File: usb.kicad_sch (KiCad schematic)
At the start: 4 parts, among them J8 MC-121-L124, U6 USBLC6-2SC6

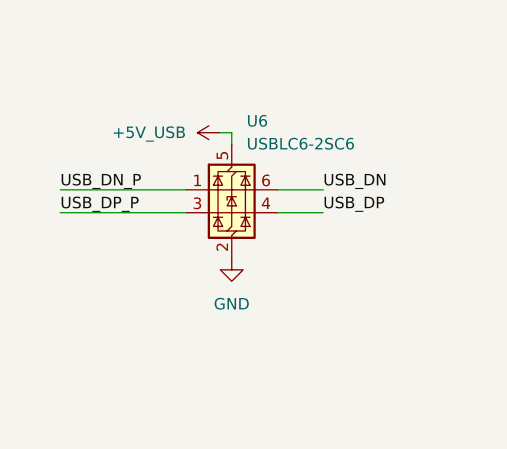
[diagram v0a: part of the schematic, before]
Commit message: Fix global nets
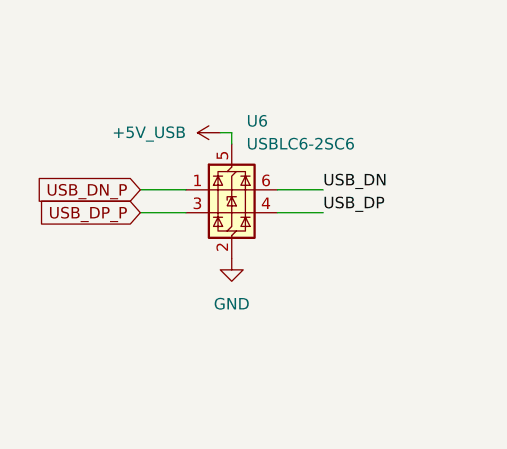
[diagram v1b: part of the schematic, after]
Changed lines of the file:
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@@
 	(wire
 		(pts
-			(xy 63.5 55.88) (xy 77.47 55.88)
+			(xy 72.39 53.34) (xy 77.47 53.34)
 		)
 		(stroke
@@
 		(pts
 			(xy 160.02 52.07) (xy 170.18 52.07)
+		)
+		(stroke
+			(width 0)
+			(type default)
+		)
+	)
+	(wire
+		(pts
+			(xy 72.39 55.88) (xy 77.47 55.88)
 		)
 		(stroke
@@
 	(wire
 		(pts
-			(xy 63.5 53.34) (xy 77.47 53.34)
-		)
-		(stroke
-			(width 0)
-			(type default)
-		)
-	)
-	(wire
-		(pts
 			(xy 168.91 69.85) (xy 168.91 67.31)
 		)
@@
 	(label "USB_DP"
 		(at 160.02 46.99 0)
-		(effects
-			(font
-				(size 1.27 1.27)
-			)
-			(justify left bottom)
-		)
-	)
-	(label "USB_DP_P"
-		(at 63.5 55.88 0)
 		(effects
 			(font
@@
 		)
 	)
-	(label "USB_DN_P"
-		(at 63.5 53.34 0)
+	(global_label "USB_DP_P"
+		(shape input)
+		(at 72.39 55.88 180)
+		(fields_autoplaced yes)
 		(effects
 			(font
 				(size 1.27 1.27)
 			)
-			(justify left bottom)
+			(justify right)
+		)
+		(property "Intersheetrefs" "${INTERSHEET_REFS}"
+			(at 59.8496 55.88 0)
+			(effects
+				(font
+					(size 1.27 1.27)
+				)
+				(justify right)
+				(hide yes)
+			)
 		)
 	)
+	(global_label "USB_DN_P"
+		(shape input)
+		(at 72.39 53.34 180)
+		(fields_autoplaced yes)
+		(effects
+			(font
+				(size 1.27 1.27)
+			)
+			(justify right)
+		)
+		(property "Intersheetrefs" "${INTERSHEET_REFS}"
+			(at 59.7891 53.34 0)
+			(effects
+				(font
+					(size 1.27 1.27)
+				)
+				(justify right)
+				(hide yes)
+			)
+		)
+	)
